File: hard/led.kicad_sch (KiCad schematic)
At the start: 0 parts

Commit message: update
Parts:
- added C19, C20, C21, C22, C23, C24, C25, C26: 100n, symbol Device:C
- added D10, D11, D12, D13, D14, D15, D16, D9: WS2812B, LED_SMD:LED_WS2812B_PLCC4_5.0x5.0mm_P3.2mm, symbol LED:WS2812B
- added R13: R, symbol Device:R
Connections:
- new net: D9.4 (DIN), R13.1
- new net +5V: C19.1, C20.1, C21.1, C22.1, C23.1, C24.1, C25.1, C26.1, D10.1 (VDD), D11.1 (VDD), D12.1 (VDD), D13.1 (VDD), D14.1 (VDD), D15.1 (VDD), D16.1 (VDD), D9.1 (VDD)
- new net DIN: R13.2
- new net GND: C19.2, C20.2, C21.2, C22.2, C23.2, C24.2, C25.2, C26.2, D10.3 (VSS), D11.3 (VSS), D12.3 (VSS), D13.3 (VSS), D14.3 (VSS), D15.3 (VSS), D16.3 (VSS), D9.3 (VSS)
- no-connect marks 0 -> 1
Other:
- note added: "DIN_INT"
- note added: "no level shifter: 3.3V -> 5V"

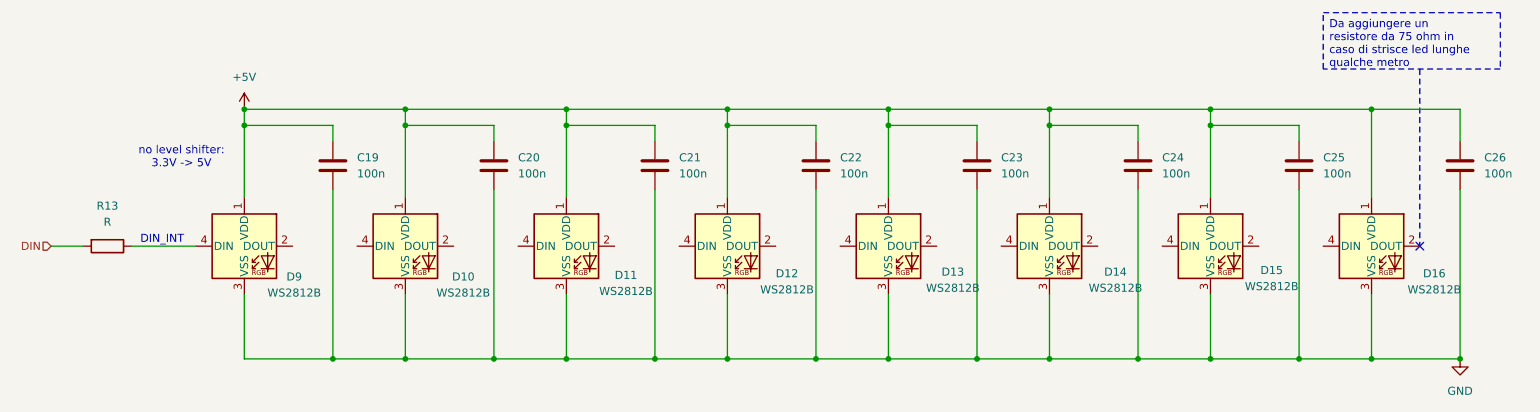
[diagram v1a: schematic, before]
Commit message: update
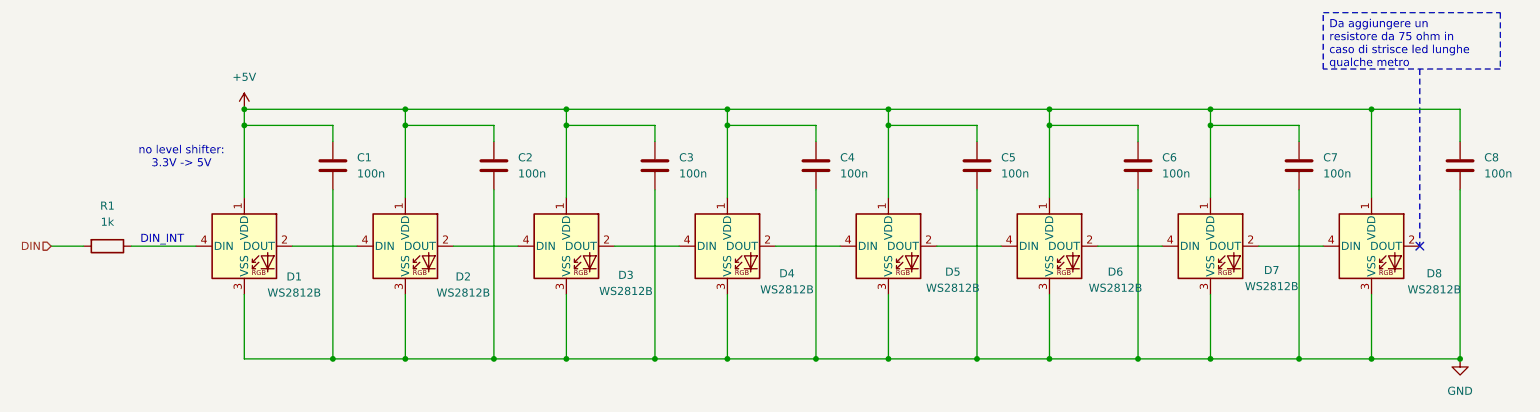
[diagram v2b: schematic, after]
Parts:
- R1: renamed from R13; value R -> 1k
- renumbered C19 to C1, C20 to C2, C21 to C3, C22 to C4, C23 to C5, C24 to C6, C25 to C7, C26 to C8, D9 to D1, D10 to D2, D11 to D3, D12 to D4, D13 to D5, D14 to D6, D15 to D7, D16 to D8
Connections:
- net at D7.2 (DOUT): now also D8.4 (DIN)
- net at D7.4 (DIN): now also D6.2 (DOUT)
- net at D6.4 (DIN): now also D5.2 (DOUT)
- net at D5.4 (DIN): now also D4.2 (DOUT)
- net at D4.4 (DIN): now also D3.2 (DOUT)
- net at D3.4 (DIN): now also D2.2 (DOUT)
- net at D2.4 (DIN): now also D1.2 (DOUT)
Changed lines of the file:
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@@
+	(wire
+		(pts
+			(xy 69.85 97.79) (xy 80.01 97.79)
+		)
+		(stroke
+			(width 0)
+			(type default)
+		)
+	)
 	(wire
 		(pts
@@
 	(wire
 		(pts
+			(xy 120.65 97.79) (xy 130.81 97.79)
+		)
+		(stroke
+			(width 0)
+			(type default)
+		)
+	)
+	(wire
+		(pts
 			(xy 113.03 76.2) (xy 113.03 78.74)
 		)
@@
 	(wire
 		(pts
+			(xy 196.85 97.79) (xy 207.01 97.79)
+		)
+		(stroke
+			(width 0)
+			(type default)
+		)
+	)
+	(wire
+		(pts
 			(xy 44.45 97.79) (xy 54.61 97.79)
 		)
@@
 	(wire
 		(pts
+			(xy 146.05 97.79) (xy 156.21 97.79)
+		)
+		(stroke
+			(width 0)
+			(type default)
+		)
+	)
+	(wire
+		(pts
+			(xy 95.25 97.79) (xy 105.41 97.79)
+		)
+		(stroke
+			(width 0)
+			(type default)
+		)
+	)
+	(wire
+		(pts
 			(xy 177.8 78.74) (xy 163.83 78.74)
 		)
@@
 	(wire
 		(pts
+			(xy 171.45 97.79) (xy 181.61 97.79)
+		)
+		(stroke
+			(width 0)
+			(type default)
+		)
+	)
+	(wire
+		(pts
 			(xy 138.43 78.74) (xy 138.43 90.17)
 		)
@@
 		(pts
 			(xy 76.2 78.74) (xy 62.23 78.74)
+		)
+		(stroke
+			(width 0)
+			(type default)
+		)
+	)
+	(wire
+		(pts
+			(xy 222.25 97.79) (xy 232.41 97.79)
 		)
 		(stroke
@@
 		(on_board yes)
 		(dnp no)
-		(property "Reference" "D15"
+		(property "Reference" "D7"
 			(at 224.282 101.6 0)
 			(effects
@@
 			(project "PSE"
 				(path "/13844229-b559-4868-a710-53f590233cb2/030c395f-3b78-4d13-857e-3ac1af28dc90"
-					(reference "D15")
+					(reference "D7")
 					(unit 1)
 				)
@@
 		(on_board yes)
 		(dnp no)
-		(property "Reference" "D14"
+		(property "Reference" "D6"
 			(at 199.644 101.854 0)
 			(effects
@@
 			(project "PSE"
 				(path "/13844229-b559-4868-a710-53f590233cb2/030c395f-3b78-4d13-857e-3ac1af28dc90"
-					(reference "D14")
+					(reference "D6")
 					(unit 1)
 				)
@@
 		(dnp no)
 		(fields_autoplaced yes)
-		(property "Reference" "C22"
+		(property "Reference" "C4"
 			(at 156.21 83.8199 0)
 			(effects
@@
 			(project "PSE"
 				(path "/13844229-b559-4868-a710-53f590233cb2/030c395f-3b78-4d13-857e-3ac1af28dc90"
-					(reference "C22")
+					(reference "C4")
 					(unit 1)
 				)
@@
 		(on_board yes)
 		(dnp no)
-		(property "Reference" "D13"
+		(property "Reference" "D5"
 			(at 173.99 101.854 0)
 			(effects
@@
 			(project "PSE"
 				(path "/13844229-b559-4868-a710-53f590233cb2/030c395f-3b78-4d13-857e-3ac1af28dc90"
-					(reference "D13")
+					(reference "D5")
 					(unit 1)
 				)
@@
 		(on_board yes)
 		(dnp no)
-		(property "Reference" "D16"
+		(property "Reference" "D8"
 			(at 249.936 102.108 0)
 			(effects
@@
 			(project "PSE"
 				(path "/13844229-b559-4868-a710-53f590233cb2/030c395f-3b78-4d13-857e-3ac1af28dc90"
-					(reference "D16")
+					(reference "D8")
 					(unit 1)
 				)
@@
 		(dnp no)
 		(fields_autoplaced yes)
-		(property "Reference" "C21"
+		(property "Reference" "C3"
 			(at 130.81 83.8199 0)
 			(effects
@@
 			(project "PSE"
 				(path "/13844229-b559-4868-a710-53f590233cb2/030c395f-3b78-4d13-857e-3ac1af28dc90"
-					(reference "C21")
+					(reference "C3")
 					(unit 1)
 				)
@@
 		(dnp no)
 		(fields_autoplaced yes)
-		(property "Reference" "R13"
+		(property "Reference" "R1"
 			(at 40.64 91.44 90)
 			(effects
@@
 			)
 		)
-		(property "Value" "R"
+		(property "Value" "1k"
 			(at 40.64 93.98 90)
 			(effects
@@
 			(project ""
 				(path "/13844229-b559-4868-a710-53f590233cb2/030c395f-3b78-4d13-857e-3ac1af28dc90"
-					(reference "R13")
+					(reference "R1")
 					(unit 1)
 				)
@@
 		(on_board yes)
 		(dnp no)
-		(property "Reference" "D12"
+		(property "Reference" "D4"
 			(at 147.828 102.108 0)
 			(effects
@@
 			(project "PSE"
 				(path "/13844229-b559-4868-a710-53f590233cb2/030c395f-3b78-4d13-857e-3ac1af28dc90"
-					(reference "D12")
+					(reference "D4")
 					(unit 1)
 				)
@@
 		(dnp no)
 		(fields_autoplaced yes)
-		(property "Reference" "C19"
+		(property "Reference" "C1"
 			(at 80.01 83.8199 0)
 			(effects
@@
 			(project ""
 				(path "/13844229-b559-4868-a710-53f590233cb2/030c395f-3b78-4d13-857e-3ac1af28dc90"
-					(reference "C19")
+					(reference "C1")
 					(unit 1)
 				)
@@
 		(on_board yes)
 		(dnp no)
-		(property "Reference" "D11"
+		(property "Reference" "D3"
 			(at 122.428 102.362 0)
 			(effects
@@
 			(project "PSE"
 				(path "/13844229-b559-4868-a710-53f590233cb2/030c395f-3b78-4d13-857e-3ac1af28dc90"
-					(reference "D11")
+					(reference "D3")
 					(unit 1)
 				)
@@
 		(on_board yes)
 		(dnp no)
-		(property "Reference" "D10"
+		(property "Reference" "D2"
 			(at 96.774 102.616 0)
 			(effects
@@
 			(project "PSE"
 				(path "/13844229-b559-4868-a710-53f590233cb2/030c395f-3b78-4d13-857e-3ac1af28dc90"
-					(reference "D10")
+					(reference "D2")
 					(unit 1)
 				)
@@
 		(dnp no)
 		(fields_autoplaced yes)
-		(property "Reference" "C20"
+		(property "Reference" "C2"
 			(at 105.41 83.8199 0)
 			(effects
@@
 			(project "PSE"
 				(path "/13844229-b559-4868-a710-53f590233cb2/030c395f-3b78-4d13-857e-3ac1af28dc90"
-					(reference "C20")
+					(reference "C2")
 					(unit 1)
 				)
@@
 		(dnp no)
 		(fields_autoplaced yes)
-		(property "Reference" "C24"
+		(property "Reference" "C6"
 			(at 207.01 83.8199 0)
 			(effects
@@
 			(project "PSE"
 				(path "/13844229-b559-4868-a710-53f590233cb2/030c395f-3b78-4d13-857e-3ac1af28dc90"
-					(reference "C24")
+					(reference "C6")
 					(unit 1)
 				)
@@
 		(dnp no)
 		(fields_autoplaced yes)
-		(property "Reference" "C26"
+		(property "Reference" "C8"
 			(at 257.81 83.8199 0)
 			(effects
@@
 			(project "PSE"
 				(path "/13844229-b559-4868-a710-53f590233cb2/030c395f-3b78-4d13-857e-3ac1af28dc90"
-					(reference "C26")
+					(reference "C8")
 					(unit 1)
 				)
@@
 		(dnp no)
 		(fields_autoplaced yes)
-		(property "Reference" "C23"
+		(property "Reference" "C5"
 			(at 181.61 83.8199 0)
 			(effects
@@
 			(project "PSE"
 				(path "/13844229-b559-4868-a710-53f590233cb2/030c395f-3b78-4d13-857e-3ac1af28dc90"
-					(reference "C23")
+					(reference "C5")
 					(unit 1)
 				)
@@
 		(on_board yes)
 		(dnp no)
-		(property "Reference" "D9"
+		(property "Reference" "D1"
 			(at 70.104 102.616 0)
 			(effects
@@
 			(project ""
 				(path "/13844229-b559-4868-a710-53f590233cb2/030c395f-3b78-4d13-857e-3ac1af28dc90"
-					(reference "D9")
+					(reference "D1")
 					(unit 1)
 				)
@@
 		(dnp no)
 		(fields_autoplaced yes)
-		(property "Reference" "C25"
+		(property "Reference" "C7"
 			(at 232.41 83.8199 0)
 			(effects
@@
 			(project "PSE"
 				(path "/13844229-b559-4868-a710-53f590233cb2/030c395f-3b78-4d13-857e-3ac1af28dc90"
-					(reference "C25")
+					(reference "C7")
 					(unit 1)
 				)

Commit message: update
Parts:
- C1, C2, C3, C4, C5, C6, C7, C8: footprint (none) -> Capacitor_Tantalum_SMD:CP_EIA-1608-08_AVX-J
- R1: footprint (none) -> Resistor_SMD:R_0201_0603Metric
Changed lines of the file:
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@@
 			)
 		)
-		(property "Footprint" ""
+		(property "Footprint" "Capacitor_Tantalum_SMD:CP_EIA-1608-08_AVX-J"
 			(at 153.3652 88.9 0)
 			(effects
@@
 			)
 		)
-		(property "Footprint" ""
+		(property "Footprint" "Capacitor_Tantalum_SMD:CP_EIA-1608-08_AVX-J"
 			(at 127.9652 88.9 0)
 			(effects
@@
 			)
 		)
-		(property "Footprint" ""
+		(property "Footprint" "Resistor_SMD:R_0201_0603Metric"
 			(at 40.64 96.012 90)
 			(effects
@@
 			)
 		)
-		(property "Footprint" ""
+		(property "Footprint" "Capacitor_Tantalum_SMD:CP_EIA-1608-08_AVX-J"
 			(at 77.1652 88.9 0)
 			(effects
@@
 			)
 		)
-		(property "Footprint" ""
+		(property "Footprint" "Capacitor_Tantalum_SMD:CP_EIA-1608-08_AVX-J"
 			(at 102.5652 88.9 0)
 			(effects
@@
 			)
 		)
-		(property "Footprint" ""
+		(property "Footprint" "Capacitor_Tantalum_SMD:CP_EIA-1608-08_AVX-J"
 			(at 204.1652 88.9 0)
 			(effects
@@
 			)
 		)
-		(property "Footprint" ""
+		(property "Footprint" "Capacitor_Tantalum_SMD:CP_EIA-1608-08_AVX-J"
 			(at 254.9652 88.9 0)
 			(effects
@@
 			)
 		)
-		(property "Footprint" ""
+		(property "Footprint" "Capacitor_Tantalum_SMD:CP_EIA-1608-08_AVX-J"
 			(at 178.7652 88.9 0)
 			(effects
@@
 			)
 		)
-		(property "Footprint" ""
+		(property "Footprint" "Capacitor_Tantalum_SMD:CP_EIA-1608-08_AVX-J"
 			(at 229.5652 88.9 0)
 			(effects
